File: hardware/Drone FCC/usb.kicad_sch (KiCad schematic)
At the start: 2 parts, among them J501 105017-0001, U501 USBLC6-2SC6

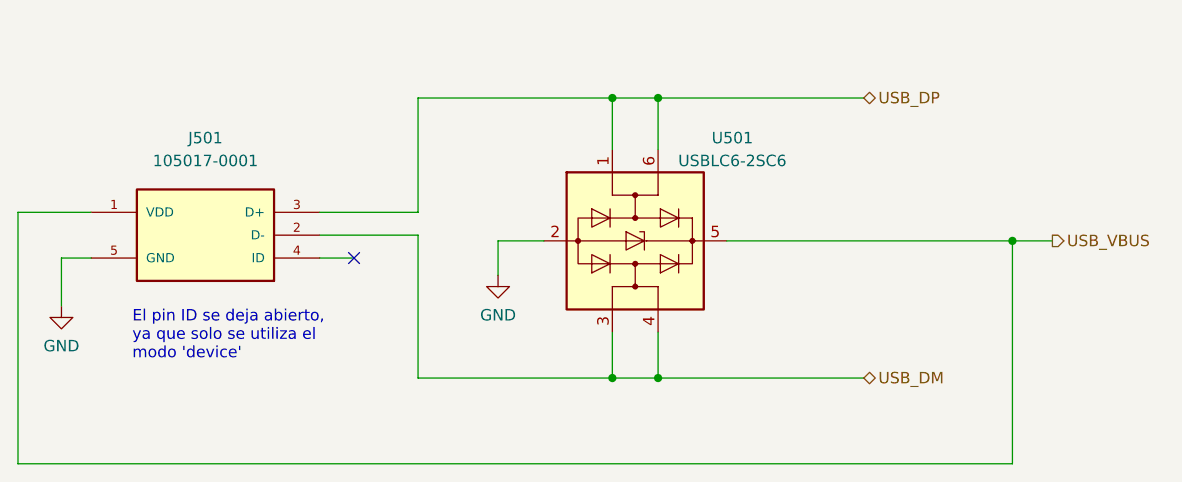
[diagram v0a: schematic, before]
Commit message: start routing
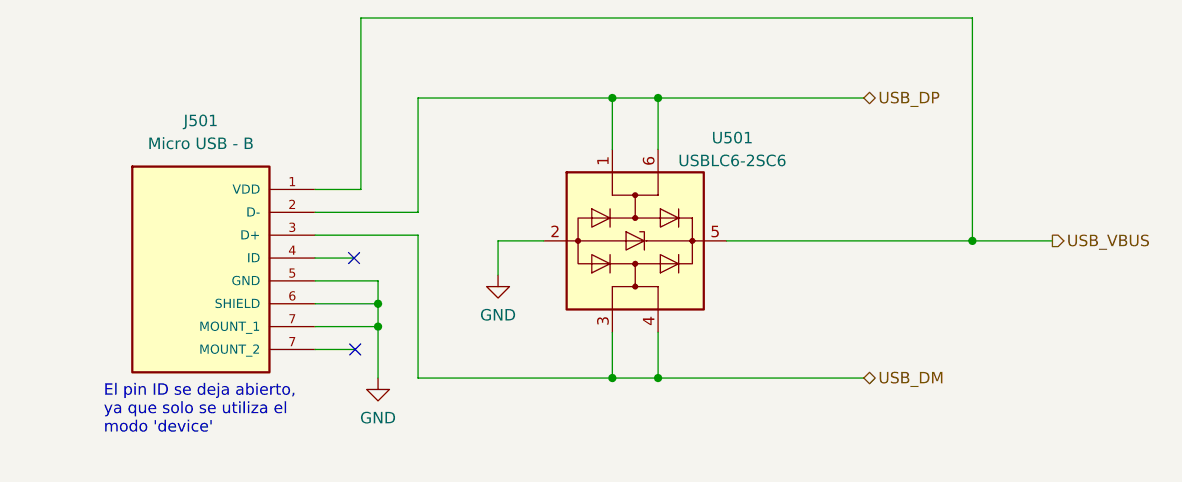
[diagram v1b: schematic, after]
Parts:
- J501: value 105017-0001 -> Micro USB - B
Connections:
- net GND: now also J501.6 (SHIELD), J501.7 (MOUNT_2)
- net USB_DM: now also J501.3 (D+); no longer J501.2 (D-)
- net USB_DP: now also J501.2 (D-); no longer J501.3 (D+)
- no-connect marks 1 -> 2
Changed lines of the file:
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@@
 (kicad_sch (version 20211123) (generator eeschema)
   (paper "A4")
+  (junction (at 168.275 89.535) (diameter 0) (color 0 0 0 0)
+  )
   (junction (at 133.35 104.775) (diameter 0) (color 0 0 0 0)
   )
   (junction (at 128.27 104.775) (diameter 0) (color 0 0 0 0)
   )
-  (junction (at 172.72 89.535) (diameter 0) (color 0 0 0 0)
+  (junction (at 133.35 73.66) (diameter 0) (color 0 0 0 0)
   )
-  (junction (at 133.35 73.66) (diameter 0) (color 0 0 0 0)
+  (junction (at 102.235 96.52) (diameter 0) (color 0 0 0 0)
+  )
+  (junction (at 102.235 99.06) (diameter 0) (color 0 0 0 0)
   )
   (junction (at 128.27 73.66) (diameter 0) (color 0 0 0 0)
   )
   (no_connect (at 99.568 91.44))
-  (wire (pts (xy 62.23 86.36) (xy 70.358 86.36))
-    (stroke (width 0) (type default) (color 0 0 0 0))
-  )
+  (no_connect (at 99.695 101.6))
   (wire (pts (xy 120.65 89.535) (xy 115.57 89.535))
     (stroke (width 0) (type default) (color 0 0 0 0))
   )
-  (wire (pts (xy 95.758 91.44) (xy 99.568 91.44))
+  (wire (pts (xy 95.25 91.44) (xy 99.568 91.44))
     (stroke (width 0) (type default) (color 0 0 0 0))
   )
@@
     (stroke (width 0) (type default) (color 0 0 0 0))
   )
+  (wire (pts (xy 100.33 83.82) (xy 100.33 64.77))
+    (stroke (width 0) (type default) (color 0 0 0 0))
+  )
   (wire (pts (xy 106.68 73.66) (xy 128.27 73.66))
     (stroke (width 0) (type default) (color 0 0 0 0))
   )
-  (wire (pts (xy 95.758 86.36) (xy 106.68 86.36))
+  (wire (pts (xy 100.33 64.77) (xy 168.275 64.77))
     (stroke (width 0) (type default) (color 0 0 0 0))
   )
-  (wire (pts (xy 95.758 88.9) (xy 106.68 88.9))
+  (wire (pts (xy 95.25 88.9) (xy 106.68 88.9))
+    (stroke (width 0) (type default) (color 0 0 0 0))
+  )
+  (wire (pts (xy 102.235 96.52) (xy 102.235 99.06))
     (stroke (width 0) (type default) (color 0 0 0 0))
   )
@@
     (stroke (width 0) (type default) (color 0 0 0 0))
   )
-  (wire (pts (xy 70.358 91.44) (xy 67.056 91.44))
+  (wire (pts (xy 95.25 86.36) (xy 106.68 86.36))
     (stroke (width 0) (type default) (color 0 0 0 0))
   )
   (wire (pts (xy 115.57 89.535) (xy 115.57 93.345))
-    (stroke (width 0) (type default) (color 0 0 0 0))
-  )
-  (wire (pts (xy 62.23 114.3) (xy 62.23 86.36))
     (stroke (width 0) (type default) (color 0 0 0 0))
   )
@@
     (stroke (width 0) (type default) (color 0 0 0 0))
   )
-  (wire (pts (xy 172.72 114.3) (xy 62.23 114.3))
+  (wire (pts (xy 95.25 96.52) (xy 102.235 96.52))
     (stroke (width 0) (type default) (color 0 0 0 0))
   )
-  (wire (pts (xy 172.72 89.535) (xy 177.165 89.535))
+  (wire (pts (xy 95.25 99.06) (xy 102.235 99.06))
+    (stroke (width 0) (type default) (color 0 0 0 0))
+  )
+  (wire (pts (xy 102.235 93.98) (xy 102.235 96.52))
+    (stroke (width 0) (type default) (color 0 0 0 0))
+  )
+  (wire (pts (xy 95.25 101.6) (xy 99.695 101.6))
     (stroke (width 0) (type default) (color 0 0 0 0))
   )
@@
     (stroke (width 0) (type default) (color 0 0 0 0))
   )
-  (wire (pts (xy 172.72 89.535) (xy 172.72 114.3))
+  (wire (pts (xy 102.235 99.06) (xy 102.235 104.775))
     (stroke (width 0) (type default) (color 0 0 0 0))
   )
-  (wire (pts (xy 67.056 91.44) (xy 67.056 96.774))
+  (wire (pts (xy 140.97 89.535) (xy 168.275 89.535))
     (stroke (width 0) (type default) (color 0 0 0 0))
   )
-  (wire (pts (xy 140.97 89.535) (xy 172.72 89.535))
+  (wire (pts (xy 168.275 89.535) (xy 177.165 89.535))
     (stroke (width 0) (type default) (color 0 0 0 0))
   )
@@
     (stroke (width 0) (type default) (color 0 0 0 0))
   )
+  (wire (pts (xy 95.25 83.82) (xy 100.33 83.82))
+    (stroke (width 0) (type default) (color 0 0 0 0))
+  )
+  (wire (pts (xy 95.25 93.98) (xy 102.235 93.98))
+    (stroke (width 0) (type default) (color 0 0 0 0))
+  )
+  (wire (pts (xy 168.275 64.77) (xy 168.275 89.535))
+    (stroke (width 0) (type default) (color 0 0 0 0))
+  )
   (text "El pin ID se deja abierto,\nya que solo se utiliza el\nmodo 'device'"
-    (at 74.93 102.87 0)
+    (at 71.755 111.125 0)
     (effects (font (size 1.27 1.27)) (justify left bottom))
   )
@@
     (pin "1")
   )
-  (symbol (lib_id "105017-0001:105017-0001") (at 83.058 88.9 0) (mirror y) (unit 1)
+  (symbol (lib_name "105017-0001_1") (lib_id "105017-0001:105017-0001") (at 82.55 95.25 0) (unit 1)
     (in_bom yes) (on_board yes) (fields_autoplaced)
-    (property "Reference" "J501" (id 0) (at 83.058 78.105 0))
-    (property "Value" "105017-0001" (id 1) (at 83.058 80.645 0))
-    (property "Footprint" "105017-0001:MOLEX_105017-0001" (id 2) (at 83.058 88.9 0)
+    (property "Reference" "J501" (id 0) (at 82.55 76.2 0))
+    (property "Value" "Micro USB - B" (id 1) (at 82.55 78.74 0))
+    (property "Footprint" "105017-0001:MOLEX_105017-0001" (id 2) (at 82.55 110.49 0)
       (effects (font (size 1.27 1.27)) (justify bottom) hide)
     )
-    (property "Datasheet" "" (id 3) (at 83.058 88.9 0)
+    (property "Datasheet" "" (id 3) (at 82.55 95.25 0)
       (effects (font (size 1.27 1.27)) hide)
     )
@@
     (pin "4")
     (pin "5")
+    (pin "6")
+    (pin "7")
+    (pin "7")
   )
-  (symbol (lib_id "power:GND") (at 67.056 96.774 0) (unit 1)
+  (symbol (lib_id "power:GND") (at 102.235 104.775 0) (mirror y) (unit 1)
     (in_bom yes) (on_board yes) (fields_autoplaced)
-    (property "Reference" "#PWR0126" (id 0) (at 67.056 103.124 0)
+    (property "Reference" "#PWR0126" (id 0) (at 102.235 111.125 0)
       (effects (font (size 1.27 1.27)) hide)
     )
-    (property "Value" "GND" (id 1) (at 67.056 101.219 0))
-    (property "Footprint" "" (id 2) (at 67.056 96.774 0)
+    (property "Value" "GND" (id 1) (at 102.235 109.22 0))
+    (property "Footprint" "" (id 2) (at 102.235 104.775 0)
       (effects (font (size 1.27 1.27)) hide)
     )
-    (property "Datasheet" "" (id 3) (at 67.056 96.774 0)
+    (property "Datasheet" "" (id 3) (at 102.235 104.775 0)
       (effects (font (size 1.27 1.27)) hide)
     )
